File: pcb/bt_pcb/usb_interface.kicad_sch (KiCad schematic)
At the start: 8 parts, among them J5 USB_C_Receptacle

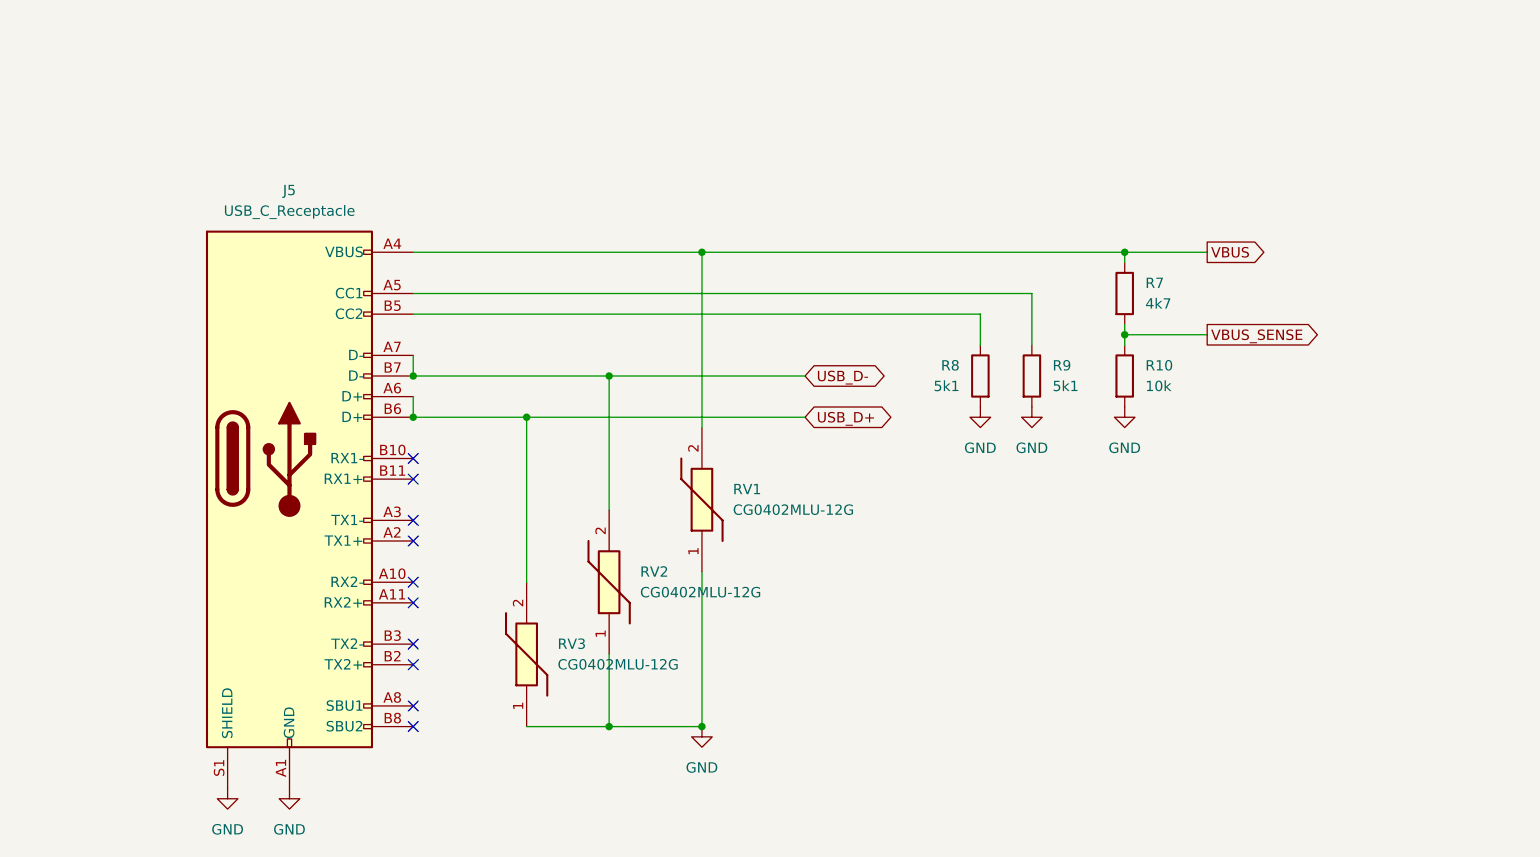
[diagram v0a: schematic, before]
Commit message: pcb started
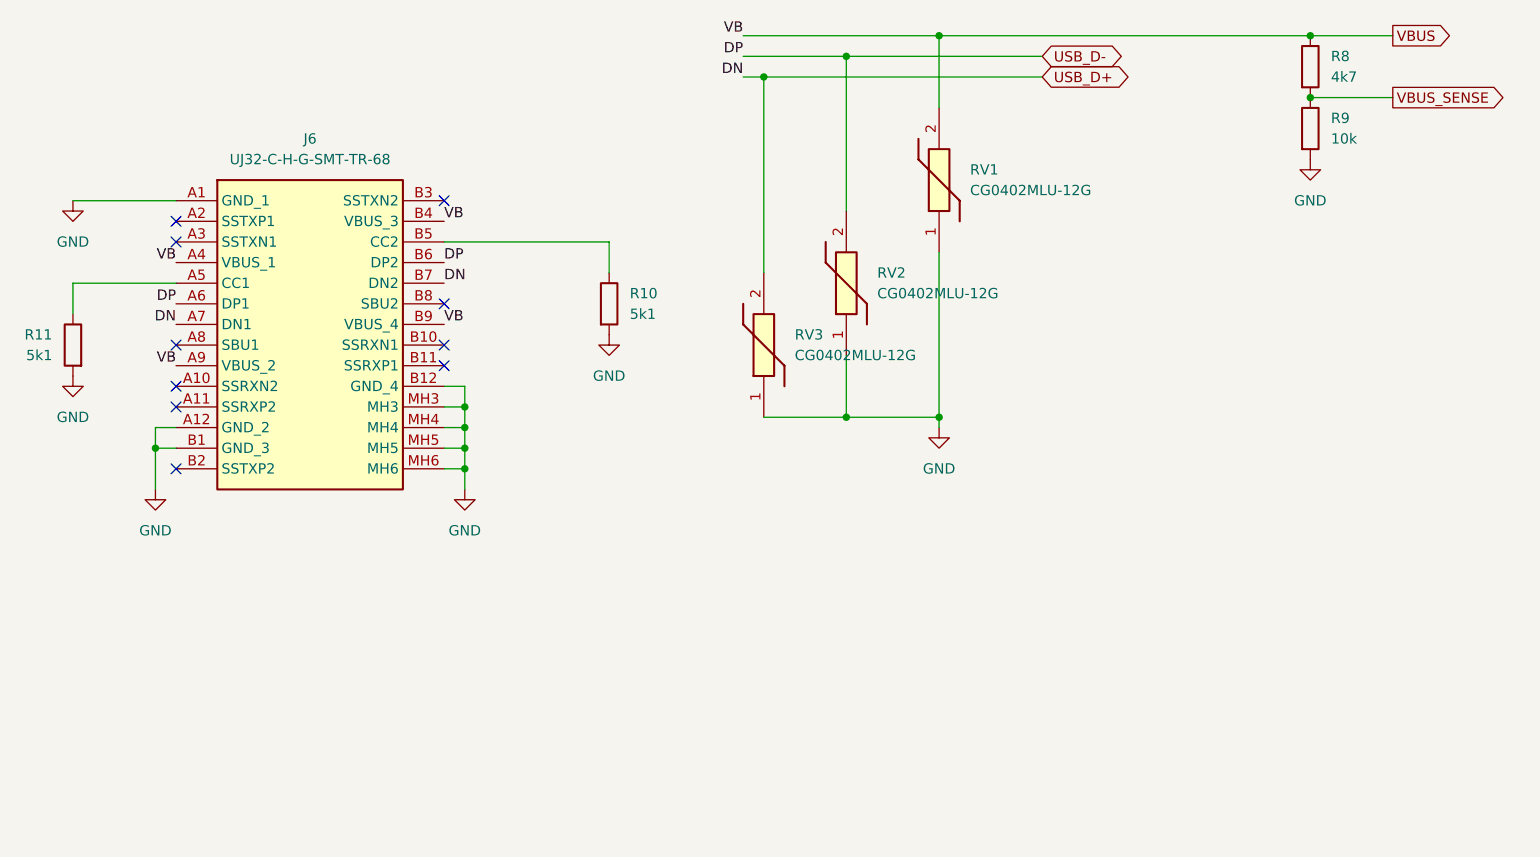
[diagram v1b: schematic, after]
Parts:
- removed J5: USB_C_Receptacle, library:UJ32CHGSMTTR68, symbol Connector:USB_C_Receptacle
- removed R8, R9: 5k1, Resistor_SMD:R_0603_1608Metric_Pad0.98x0.95mm_HandSolder, symbol Device:R
- added J6: UJ32-C-H-G-SMT-TR-68, library:UJ32CHGSMTTR68, symbol library:UJ32-C-H-G-SMT-TR-68
- added R10, R11: 5k1, Resistor_SMD:R_0603_1608Metric_Pad0.98x0.95mm_HandSolder, symbol Device:R
- renumbered R7 to R8, R10 to R9
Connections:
- net GND: now also J6.A1 (GND_1), J6.A12 (GND_2), J6.B1 (GND_3), J6.B12 (GND_4), J6.MH3, J6.MH4, J6.MH5, J6.MH6, R10.2, R11.2
- net USB_D+: now also J6.A7 (DN1), J6.B7 (DN2)
- net USB_D-: now also J6.A6 (DP1), J6.B6 (DP2)
- net VBUS: now also J6.A4 (VBUS_1), J6.A9 (VBUS_2), J6.B4 (VBUS_3), J6.B9 (VBUS_4)
- new net: J6.A5 (CC1), R11.1
- new net: J6.B5 (CC2), R10.1
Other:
- moved on the sheet: R8, R9, RV1, RV2, RV3
